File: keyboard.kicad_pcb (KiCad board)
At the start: 2 copper layers, 75.4 x 113.7 mm, 122 parts, among them IC1 ATMEGA32U4, J1 MINI, M1 HOLE, M10 HOLE, M11 HOLE, M12 HOLE, M13 HOLE, M14 HOLE, M15 HOLE, M16 HOLE, M17 HOLE, M2 HOLE, M3 HOLE, M4 HOLE, M5 HOLE, M6 HOLE, M7 HOLE, M8 HOLE, M9 HOLE, P1 MISO, P10 ROW4, P11 ROW5, P12 ROW6, P13 COL1, P14 COL2, P15 COL3, P16 COL4, P17 FNLED, P18 Vcc, P19 GND, P2 Vcc, P200 GND, P201 GND, P202 GND, P203 GND, P204 GND, P205 GND, P3 SCK, P4 MOSI, P5 RES, P6 GND, P7 ROW1, P8 ROW2, P9 ROW3, X1 ASX3F

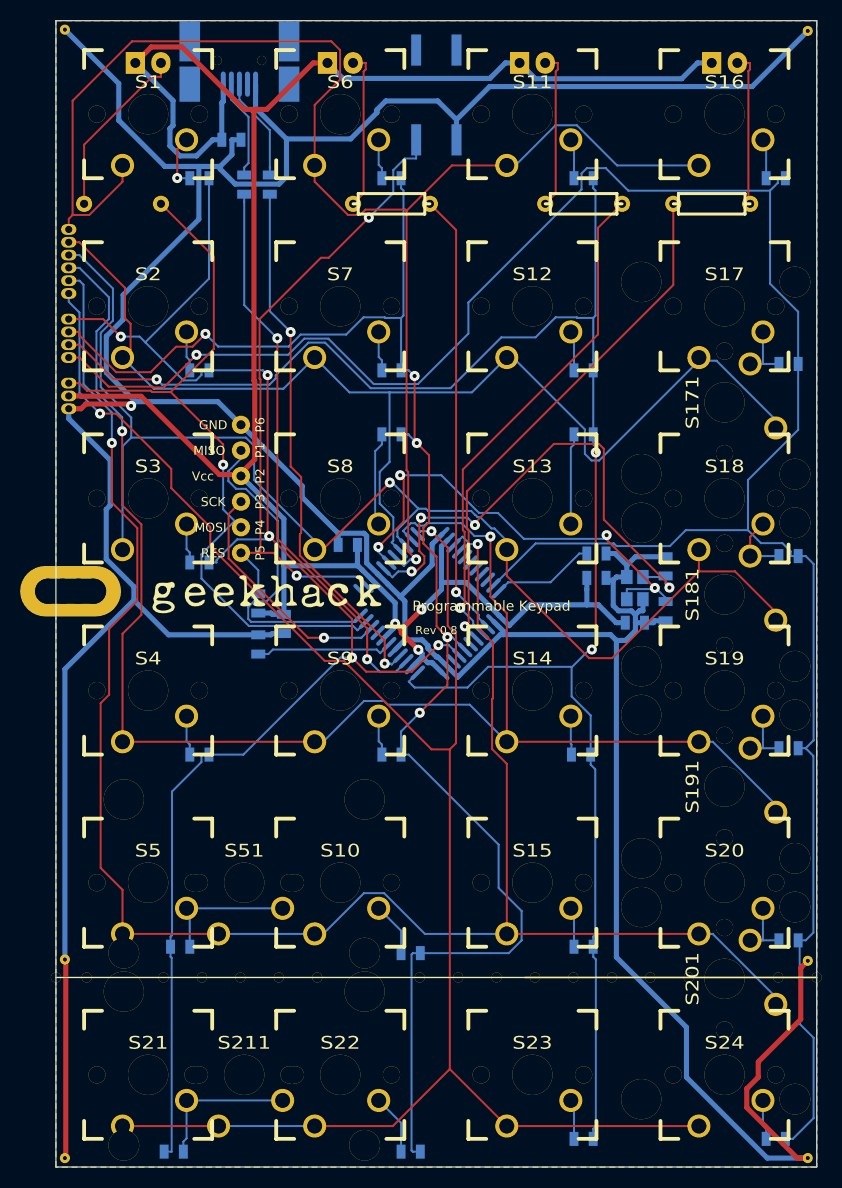
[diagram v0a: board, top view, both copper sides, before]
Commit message: v0.9
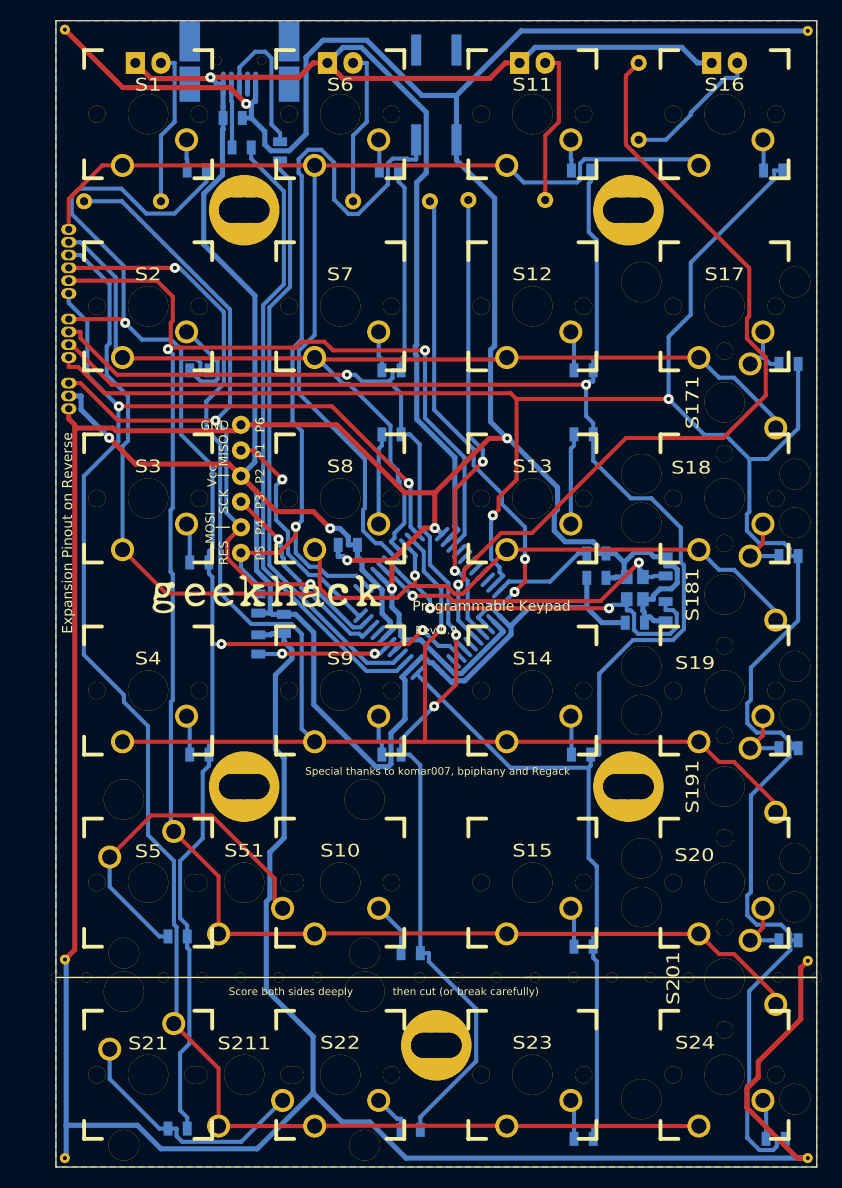
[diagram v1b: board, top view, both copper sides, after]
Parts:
- added H1: HOLE, Mechanical_Slotted_Hole, F.Cu at (81.0, 83.3)
- added H3: HOLE, Mechanical_Slotted_Hole, F.Cu at (81.0, 140.5)
- added H4: HOLE, Mechanical_Slotted_Hole, F.Cu at (119.1, 140.5)
- added H5: HOLE, Mechanical_Slotted_Hole, F.Cu at (100.0, 166.1)
- H2: footprint Mechanical_Slot -> Mechanical_Slotted_Hole
- RF1, RF2, RF3: moved to B.Cu
- moved H2 67.0 mm to (119.1, 83.3)
- moved RF3 12.5 mm to (120.1, 72.5), turned to 270 degrees
- moved RF2 7.63 mm to (107.0, 82.3), turned to 0 degrees
- moved R1 3.69 mm to (80.7, 77.1), turned to 180 degrees
- moved R2 3.45 mm to (84.5, 77.5)
- moved D21 2.32 mm to (74.4, 174.4), turned to 180 degrees
- moved C8 2.16 mm to (79.8, 74.2)
- moved D22 2.16 mm to (97.5, 174.5)
- moved D5 1.05 mm to (74.4, 155.4), turned to 0 degrees
- moved D16 0.80 mm to (133.4, 79.4)
- moved D1 0.80 mm to (76.3, 79.4)
- moved D11 0.80 mm to (114.4, 79.4)
- moved D6 0.80 mm to (95.3, 79.4)
- moved R4 0.25 mm to (68.9, 82.5), turned to 180 degrees
- moved RF1 0.25 mm to (95.6, 82.5)
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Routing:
- net GND: track 426.0 -> 497.6 mm, vias 1 -> 5
- net VCC: track 224.0 -> 290.8 mm
- net /Matrix/row1: track 146.9 -> 113.6 mm, vias 1 -> 0
- net /GPIO2: track 52.3 -> 84.3 mm
- net N-0000054: track 13.3 -> 34.7 mm
- net N-0000020: track 51.9 -> 32.4 mm, vias 4 -> 2
- net /Matrix/col2: track 160.1 -> 144.5 mm, vias 5 -> 3
- net /~RES~: track 67.1 -> 82.7 mm, vias 2 -> 1
- net /Matrix/row3: track 129.9 -> 114.5 mm
- net /MISO: track 33.3 -> 23.2 mm, vias 0 -> 1
- net N-0000051: track 14.7 -> 24.8 mm
- net N-0000037: track 46.4 -> 37.8 mm, vias 4 -> 2
- net /Matrix/row2: track 115.6 -> 107.0 mm
- net /Matrix/col3: track 176.8 -> 183.7 mm, vias 3 -> 1
- net N-0000019: track 56.0 -> 62.7 mm, vias 2 -> 0
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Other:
- board text added: "Expansion Pinout on Reverse"
- board text added: "FOR S1 LED"
- board text added: "FOR S11 LED"
- board text added: "FOR S16 LED"
- board text added: "FOR S6 LED"
- board text added: "Rev 0.9"
- board text added: "S1"
- board text added: "S11"
- board text added: "S16"
- board text added: "S1LED"
- board text added: "S6"
- board text added: "Score both sides deeply then cut (or break carefully)"
- board text added: "Special thanks to komar007, bpiphany and Regack"
- board text added: "or D171"
- board text added: "or D181"
- board text added: "or D191"
- board text added: "or D201"
- board text added: "orD211"
- board text added: "orD51"
- board text removed: "CAPS"
- board text removed: "ESC"
- board text removed: "Rev 0.8"
